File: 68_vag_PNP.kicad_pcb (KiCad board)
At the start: 2 copper layers, 154 x 159 mm, 173 parts, among them J1 Conn_01x01, J10 Conn_02x11_Odd_Even, J11 Conn_02x11_Odd_Even, J12 Conn_02x11_Odd_Even, J13 Conn_02x11_Odd_Even, J14 Conn_02x11_Odd_Even, J15 Conn_02x11_Odd_Even, J16 Conn_02x11_Odd_Even, J17 Conn_02x11_Odd_Even, J18 Conn_02x11_Odd_Even, J19 Conn_02x11_Odd_Even, J2 Conn_01x01, J20 Conn_02x11_Odd_Even, J21 Conn_02x11_Odd_Even, J22 Conn_02x11_Odd_Even, J23 Conn_02x11_Odd_Even, J24 Conn_01x01, J25 Conn_01x01, J26 Conn_01x01, J27 Conn_01x01, J28 Conn_01x01, J29 Conn_01x01, J3 Conn_01x01, J30 Conn_01x01, J31 Conn_01x01, J32 Conn_01x01, J33 Conn_01x01, J34 Conn_01x01, J35 Conn_01x01, J36 Conn_01x01, J37 Conn_01x01, J38 Conn_01x01, J39 Conn_01x01, J4 Conn_01x05, J40 Conn_01x01, J5 Conn_01x01, J6 Conn_01x05, J7 Conn_01x05, J8 Conn_01x05, J9 Conn_02x11_Odd_Even, P1 1123038-2, U1 VNLD5090, U2 VNLD5090, U3 molex_48pin_MRE, U4 ITEAD_HC-05

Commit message: draft
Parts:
- moved BT1 261.9 mm to (418.5, 128.9)
- moved C1 261.9 mm to (306.8, 73.2)
- moved C2 261.9 mm to (306.8, 76.3)
- moved C3 261.9 mm to (306.8, 86.4)
- moved C4 261.9 mm to (306.8, 89.7)
- moved C5 261.9 mm to (307.4, 128.6)
- moved D16 261.9 mm to (315.0, 61.7)
- moved D2 261.9 mm to (309.1, 77.3)
- moved D20 261.9 mm to (318.9, 61.7)
- moved D21 261.9 mm to (323.3, 57.8)
- moved D22 261.9 mm to (323.3, 61.7)
- moved D27 261.9 mm to (335.4, 57.7)
- moved D28 261.9 mm to (335.4, 61.7)
- moved D30 261.9 mm to (377.6, 48.9)
- moved D5 261.9 mm to (309.1, 84.1)
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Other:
- board size 154 x 159 mm -> 149 x 85 mm

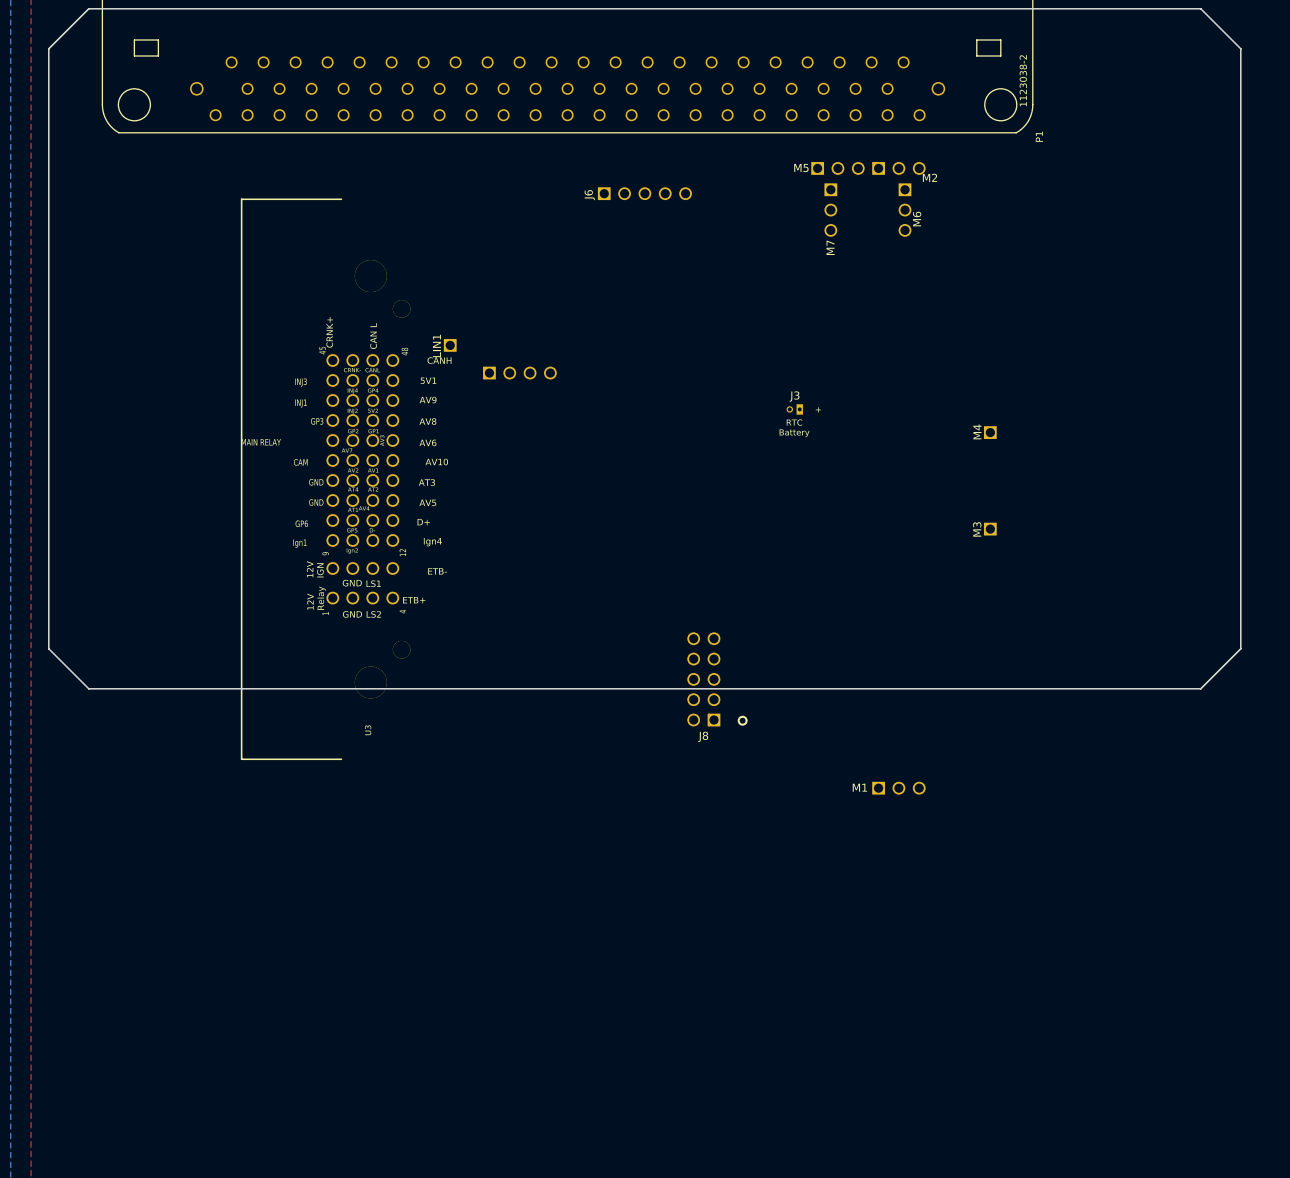
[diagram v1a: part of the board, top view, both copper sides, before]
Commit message: draft
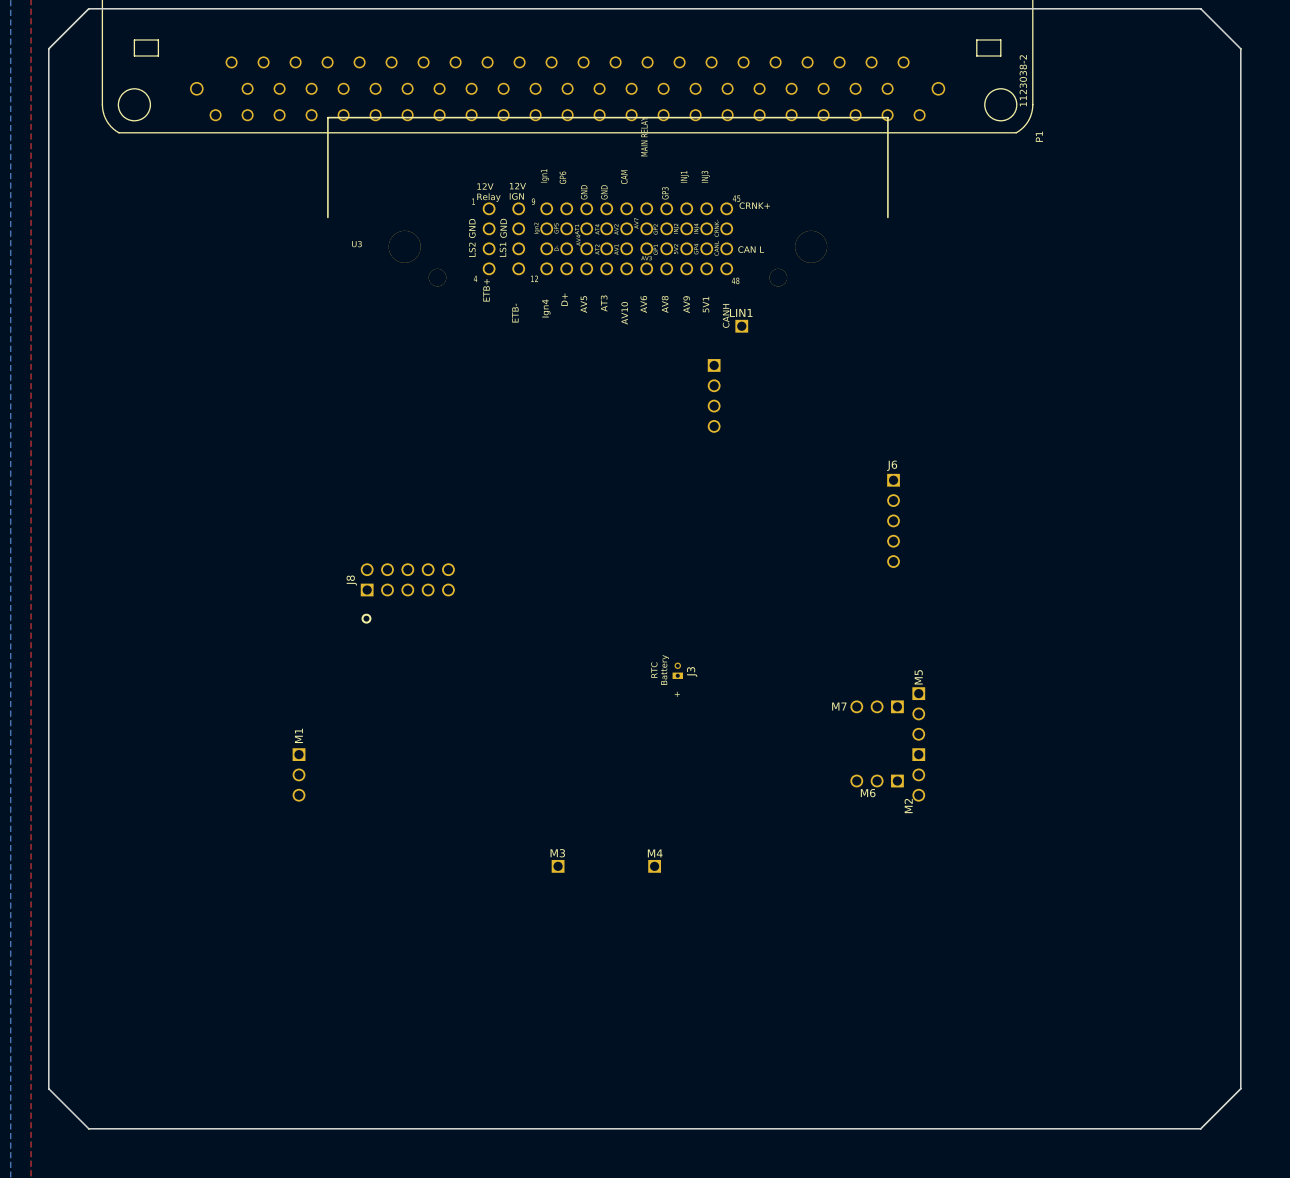
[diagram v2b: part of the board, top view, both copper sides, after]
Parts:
- moved U3 52.5 mm to (75.0, 45.0), turned to 0 degrees
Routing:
- net GND: vias 123 -> 122
- net (no net): vias 1 -> 2
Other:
- board size 149 x 85 mm -> 149 x 140 mm
